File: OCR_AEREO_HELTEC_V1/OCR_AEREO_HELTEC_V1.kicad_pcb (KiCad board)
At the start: 2 copper layers, 120.5 x 108 mm, 25 parts, among them J1 Conn_01x04_Socket, J10 Conn_01x02_Pin, J11 Conn_01x02_Pin, J12 Conn_01x08_Socket, J14 MODULO SD, J19 BIOSHUT, J2 Conn_01x04_Socket, J3 Conn_01x18_Pin, J4 Conn_01x02_Pin, J5 Conn_01x02_Pin, J6 OCR, J7 BATERÍA, J8 Conn_01x02_Pin, J9 Conn_01x02_Pin, U2 MAX3232

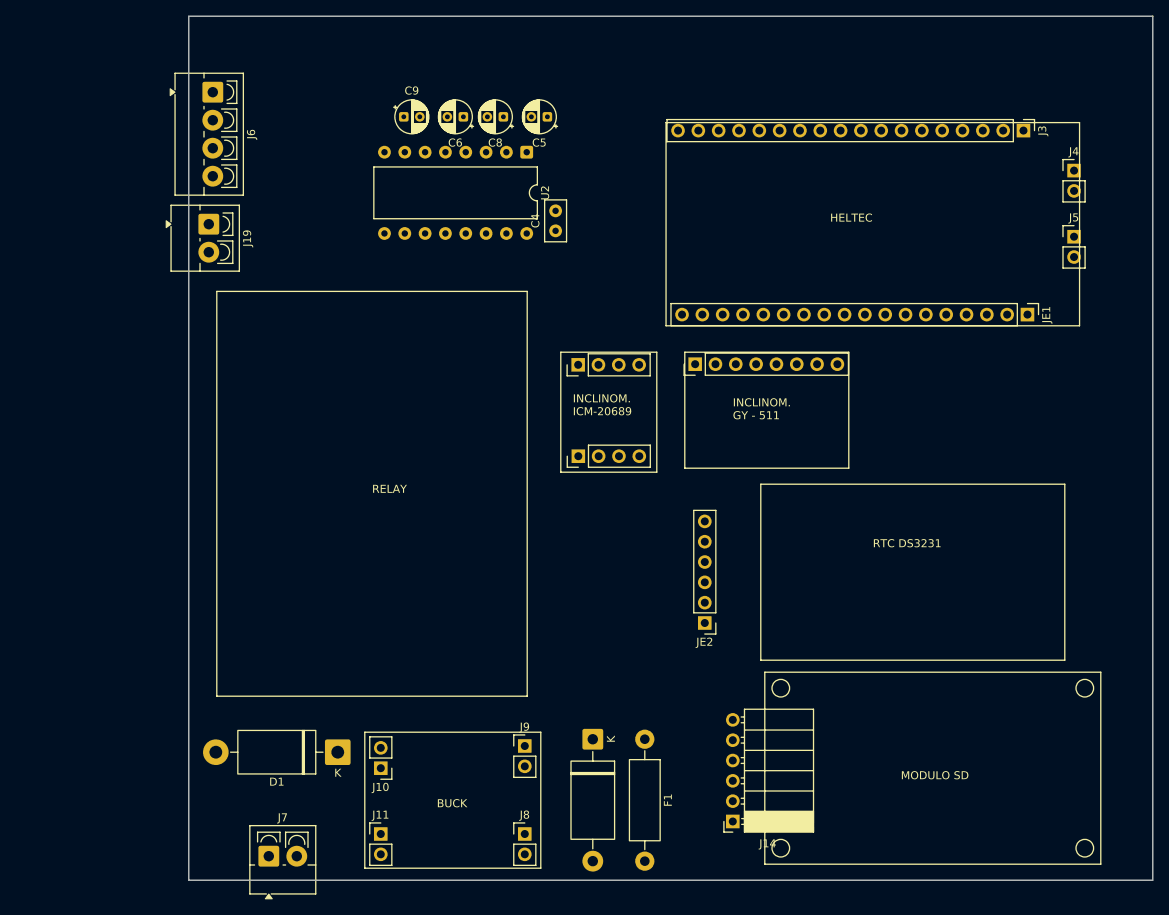
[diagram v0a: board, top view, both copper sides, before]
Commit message: actualizacion V2
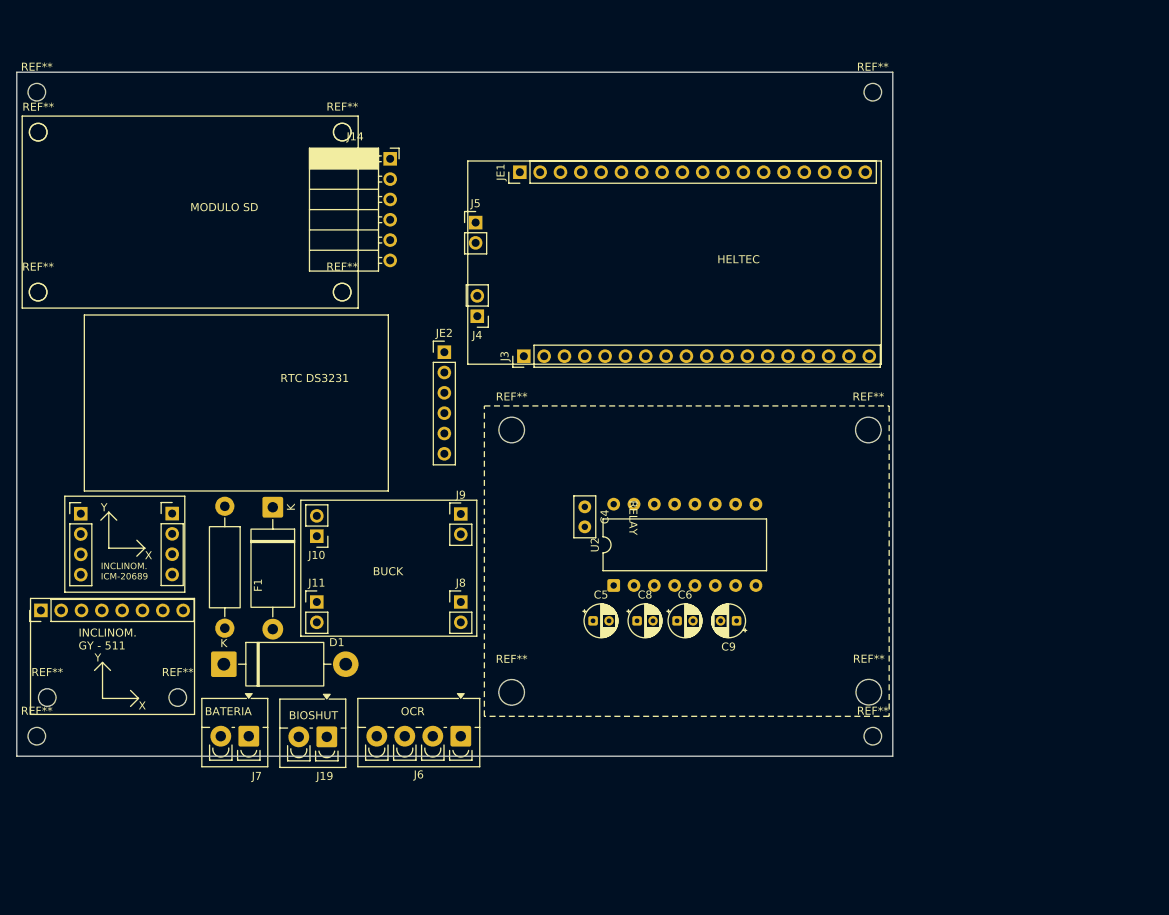
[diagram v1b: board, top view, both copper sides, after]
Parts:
- added REF**: MountingHole_2.2mm_M2, MountingHole:MountingHole_2.2mm_M2, F.Cu at (42.7, 47.5)
- added REF**: MountingHole_2.2mm_M2, MountingHole:MountingHole_2.2mm_M2, F.Cu at (42.5, 42.5)
- added REF**: MountingHole_2.2mm_M2, MountingHole:MountingHole_2.2mm_M2, F.Cu at (43.8, 118.2)
- added REF**: MountingHole_2.2mm_M2, MountingHole:MountingHole_2.2mm_M2, F.Cu at (147.0, 123.0)
- added REF**: MountingHole_3.2mm_M3, MountingHole:MountingHole_3.2mm_M3, F.Cu at (101.9, 117.5)
- added REF**: MountingHole_2.2mm_M2, MountingHole:MountingHole_2.2mm_M2, F.Cu at (80.7, 67.5)
- added REF**: MountingHole_2.2mm_M2, MountingHole:MountingHole_2.2mm_M2, F.Cu at (60.1, 118.2)
- added REF**: MountingHole_3.2mm_M3, MountingHole:MountingHole_3.2mm_M3, F.Cu at (146.4, 84.7)
- added REF**: MountingHole_2.2mm_M2, MountingHole:MountingHole_2.2mm_M2, F.Cu at (147.0, 42.5)
- added REF**: MountingHole_3.2mm_M3, MountingHole:MountingHole_3.2mm_M3, F.Cu at (101.9, 84.7)
- added REF**: MountingHole_3.2mm_M3, MountingHole:MountingHole_3.2mm_M3, F.Cu at (146.5, 117.5)
- added REF**: MountingHole_2.2mm_M2, MountingHole:MountingHole_2.2mm_M2, F.Cu at (80.7, 47.5)
- added REF**: MountingHole_2.2mm_M2, MountingHole:MountingHole_2.2mm_M2, F.Cu at (42.5, 123.0)
- added REF**: MountingHole_2.2mm_M2, MountingHole:MountingHole_2.2mm_M2, F.Cu at (42.7, 67.5)
- moved J14 93.2 mm to (86.7, 50.8), turned to 0 degrees
- moved J12 87.4 mm to (43.0, 107.3)
- moved J6 86.3 mm to (95.5, 123.0), turned to 180 degrees
- moved J4 76.8 mm to (97.6, 70.5), turned to 180 degrees
- moved C9 75.5 mm to (130.0, 108.6), turned to 180 degrees
- moved J5 74.8 mm to (97.4, 58.8)
- moved J3 68.5 mm to (103.4, 75.5), turned to 90 degrees
- moved C6 68.4 mm to (122.5, 108.6), turned to 0 degrees
- moved JE1 65.9 mm to (102.9, 52.5), turned to 90 degrees
- moved J19 65.8 mm to (78.8, 123.1), turned to 180 degrees
- moved C8 65.2 mm to (117.5, 108.6), turned to 0 degrees
- moved C5 63.3 mm to (112.0, 108.6), turned to 0 degrees
- moved J1 62.6 mm to (48.0, 95.2), turned to 0 degrees
- moved F1 60.0 mm to (66.0, 94.3)
- moved U2 55.2 mm to (114.6, 104.2), turned to 90 degrees
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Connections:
- J12 pad 2: INT_INCL -> INT_INCL_2
- J2 pad 1: INT_INCL -> INT_INCL_1
- J3 pad 5: INT_INCL -> INT_INCL_1
- J3 pad 6: unconnected-(J3-Pin_6-Pad6) -> INT_INCL_2
- J5 pad 1: unconnected-(J5-Pin_1-Pad1) -> SDA
- J5 pad 2: unconnected-(J5-Pin_2-Pad2) -> SCL
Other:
- board size 120.5 x 108 mm -> 109.5 x 85.5 mm
- board text added: "BATERIA"
- board text added: "BIOSHUT"
- board text added: "OCR"
- board text added: "X"
- board text added: "Y"
